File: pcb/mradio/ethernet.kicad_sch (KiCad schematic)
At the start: 28 parts, among them J1 JX0026D21BNL, U2 DP83825I, Y301 DSC1525JL2A-25M00000T

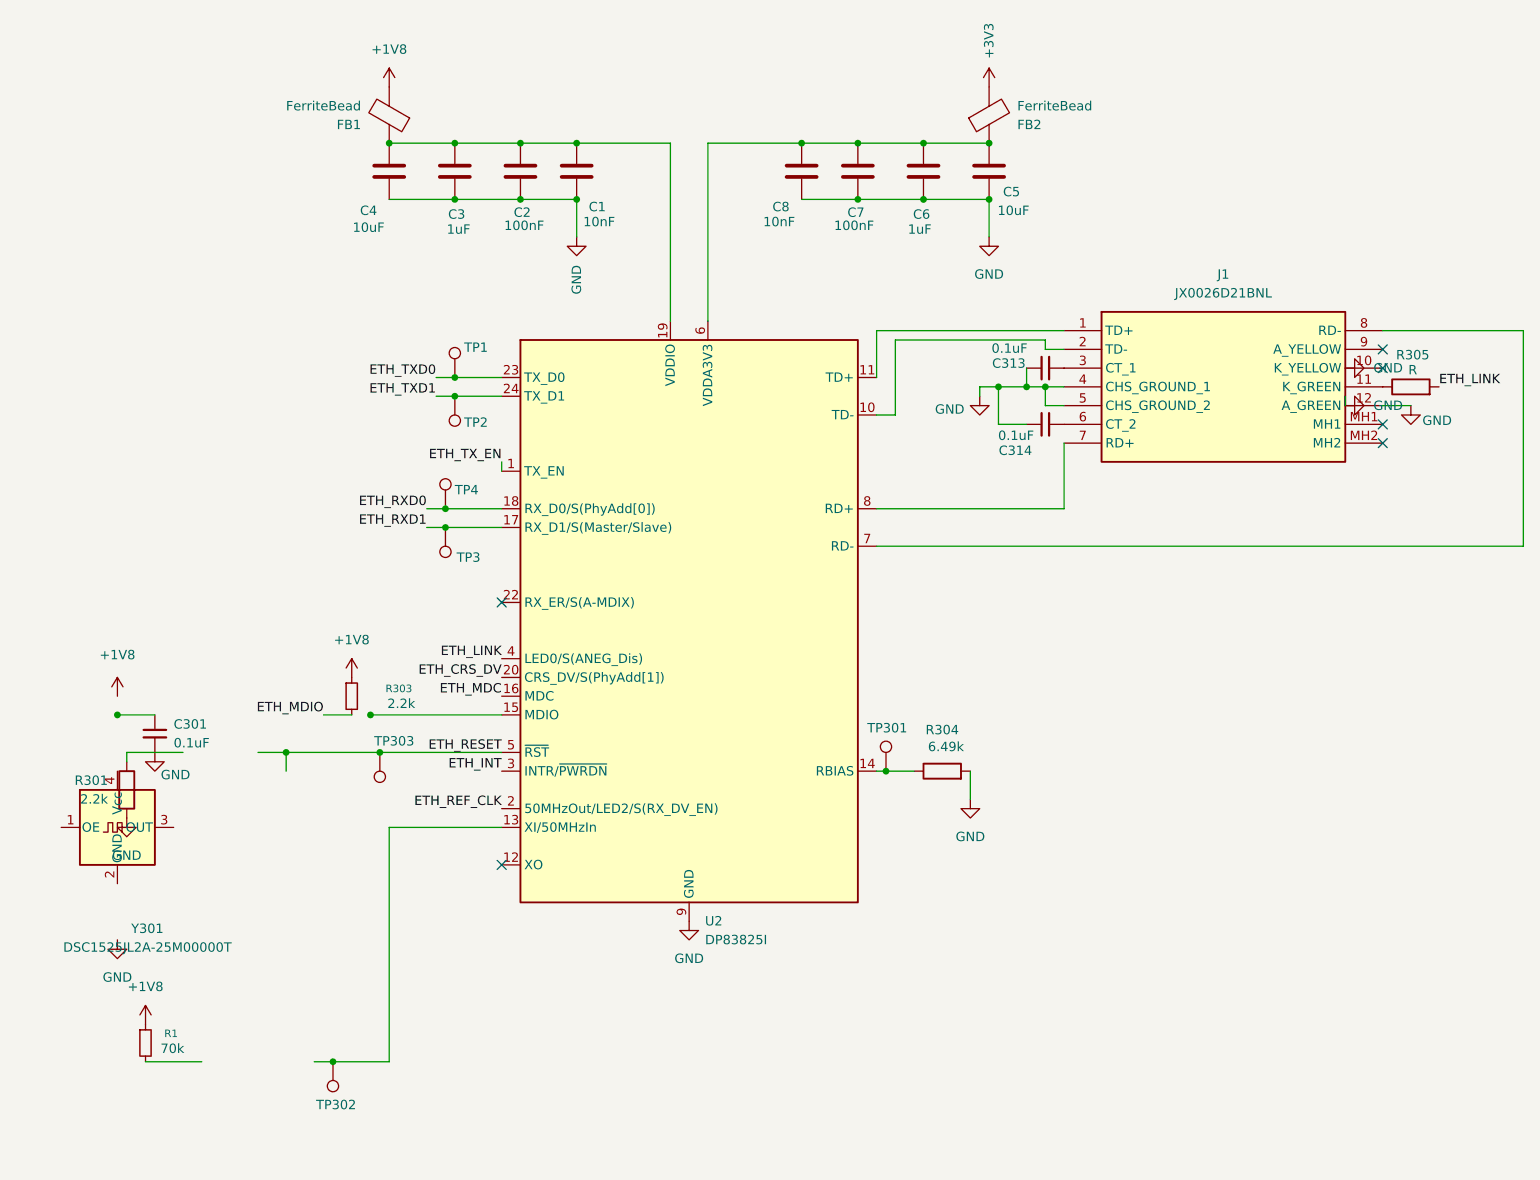
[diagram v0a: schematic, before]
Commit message: ethernet oscillator
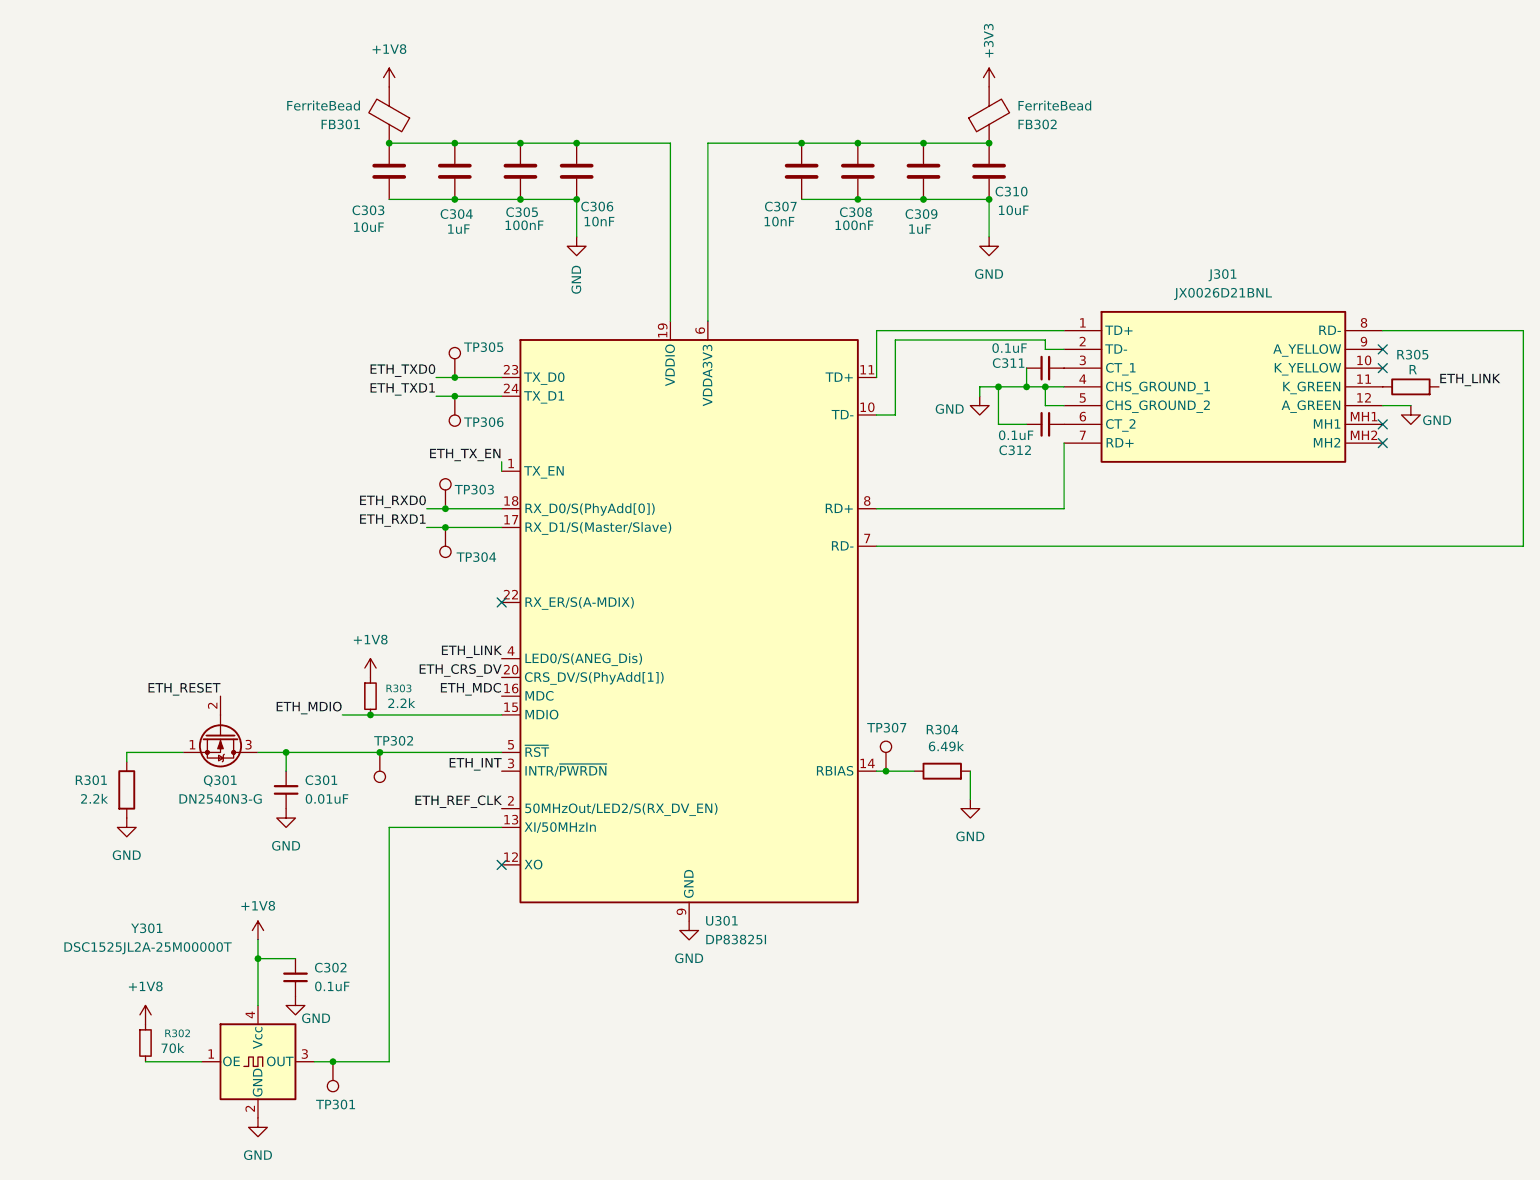
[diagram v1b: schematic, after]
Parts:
- added C301: 0.01uF, symbol Device:C_Small
- added Q301: DN2540N3-G, Package_TO_SOT_THT:TO-92_Inline, symbol Transistor_FET_Other:DN2540N3-G
- renumbered C301 to C302, C4 to C303, C3 to C304, C2 to C305, C1 to C306, C8 to C307, C7 to C308, C6 to C309, C5 to C310, C313 to C311, C314 to C312, FB1 to FB301, FB2 to FB302, J1 to J301, R1 to R302, TP302 to TP301, TP303 to TP302, TP4 to TP303, TP3 to TP304, TP1 to TP305, TP2 to TP306, TP301 to TP307, U2 to U301
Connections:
- net +1V8: now also C302.1, Y301.4 (Vcc)
- net ETH_MDIO: now also U301.15 (MDIO)
- net ETH_RESET: now also Q301.2 (G); no longer TP302.1, U301.5 (~{RST})
- net GND: now also Y301.2 (GND), C301.2
- net at R302.2: now also Y301.1 (OE)
- net at TP301.1, U301.13 (XI/50MHzIn): now also Y301.3 (OUT)
- net at R301.1: now also Q301.1 (S)
- new net: C301.1, Q301.3 (D), TP302.1, U301.5 (~{RST})
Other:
- moved on the sheet: C302, R303, Y301

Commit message: Fixed numbers
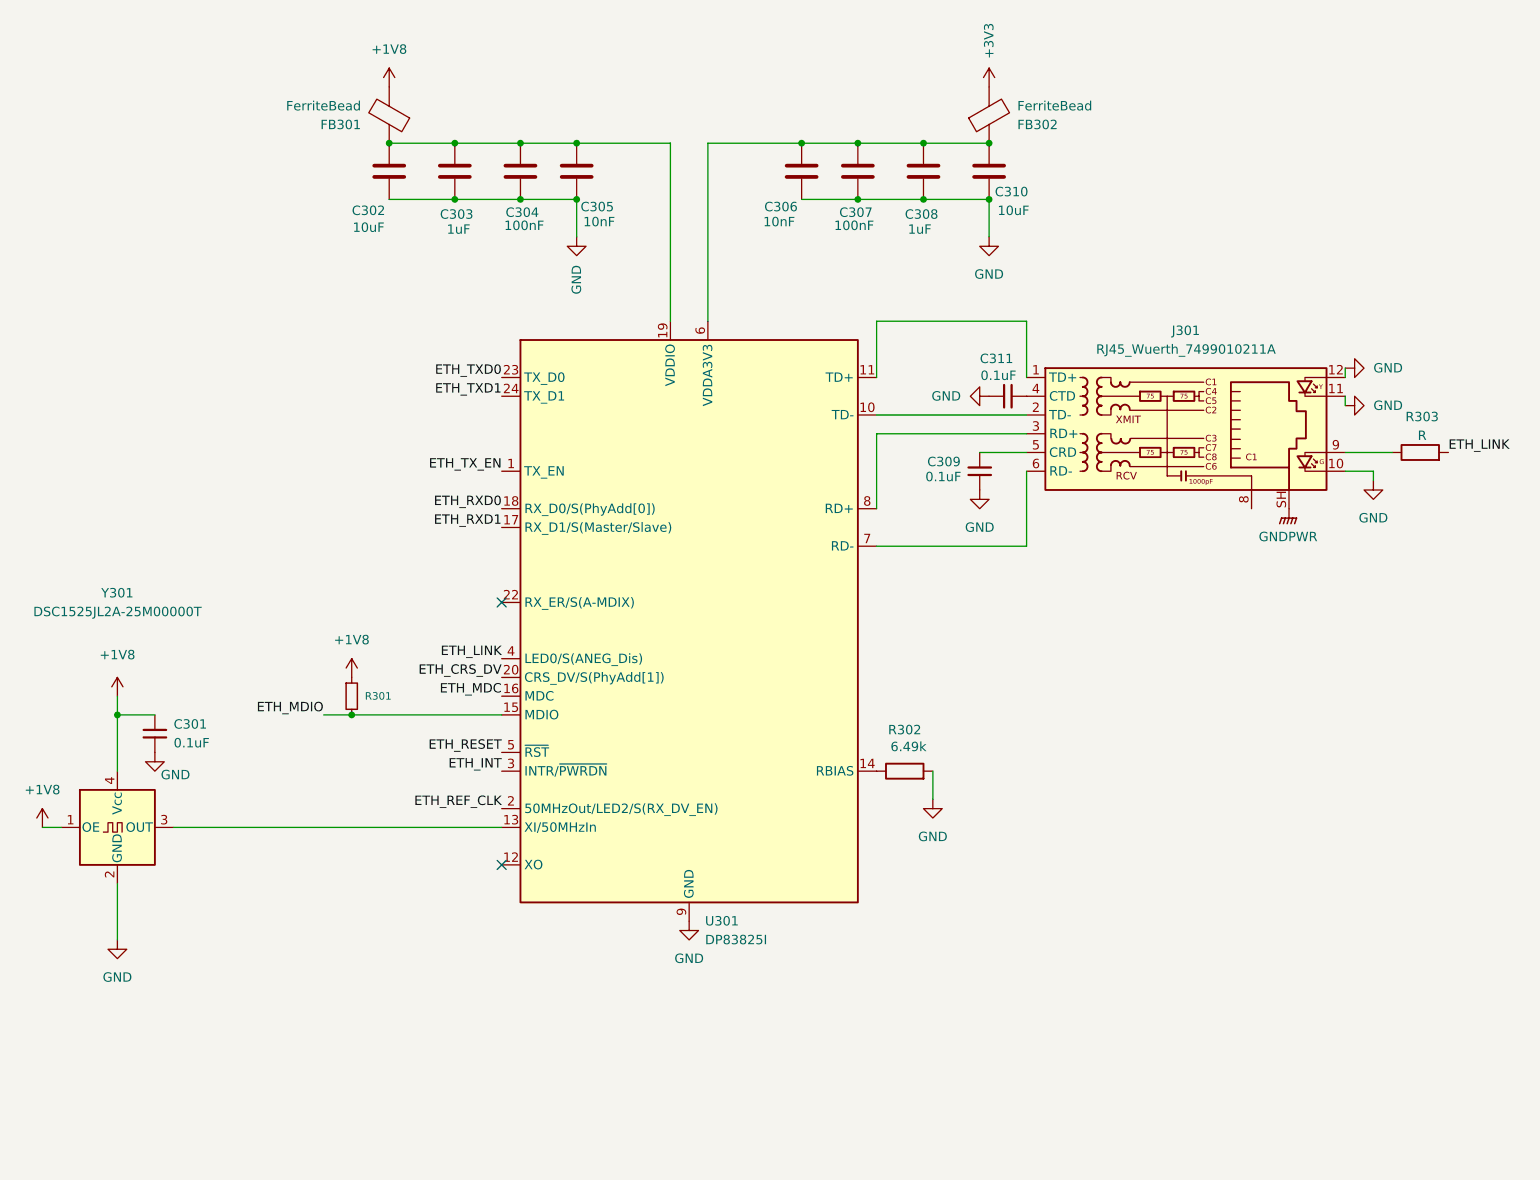
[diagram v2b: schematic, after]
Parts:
- removed C301: 0.01uF, symbol Device:C_Small
- removed C312: 0.1uF, symbol Device:C_Small
- removed J301: JX0026D21BNL, JX0026D21BNL:JX0026D21BNL, symbol symbols:JX0026D21BNL
- removed Q301: DN2540N3-G, Package_TO_SOT_THT:TO-92_Inline, symbol Transistor_FET_Other:DN2540N3-G
- removed R301: 2.2k, Package_TO_SOT_THT:TO-92_Inline, symbol Device:R
- removed R302: 70k, symbol Device:R_Small
- removed R305: R, symbol Device:R
- removed TP301, TP302, TP303, TP304, TP305, TP306, TP307: TestPoint, symbol Connector:TestPoint
- added C309: 0.1uF, symbol Device:C_Small
- added J301: RJ45_Wuerth_7499010211A, Connector_RJ:RJ45_Wuerth_7499010211A_Horizontal, symbol Connector:RJ45_Wuerth_7499010211A
- added R303: R, symbol Device:R
- R301: renamed from R303; value 2.2k -> (none)
- renumbered C302 to C301, C303 to C302, C304 to C303, C305 to C304, C306 to C305, C307 to C306, C308 to C307, C309 to C308, R304 to R302
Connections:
- net +1V8: now also Y301.1 (OE)
- net ETH_LINK: now also R303.2
- net ETH_RESET: now also U301.5 (~{RST})
- net GND: now also C309.2, J301.10, J301.11, J301.12
- net at U301.11 (TD+): now also J301.1 (TD+)
- net at U301.10 (TD-): now also J301.2 (TD-)
- net at C311.2: now also J301.4 (CTD)
- net at U301.8 (RD+): now also J301.3 (RD+)
- net at U301.7 (RD-): now also J301.6 (RD-)
- new net: C309.1, J301.5 (CRD)
- new net: J301.9, R303.1
- new net GNDPWR: J301.SH
- no-connect marks 6 -> 2
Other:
- moved on the sheet: C301, R301, R302, Y301

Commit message: undid overwrite
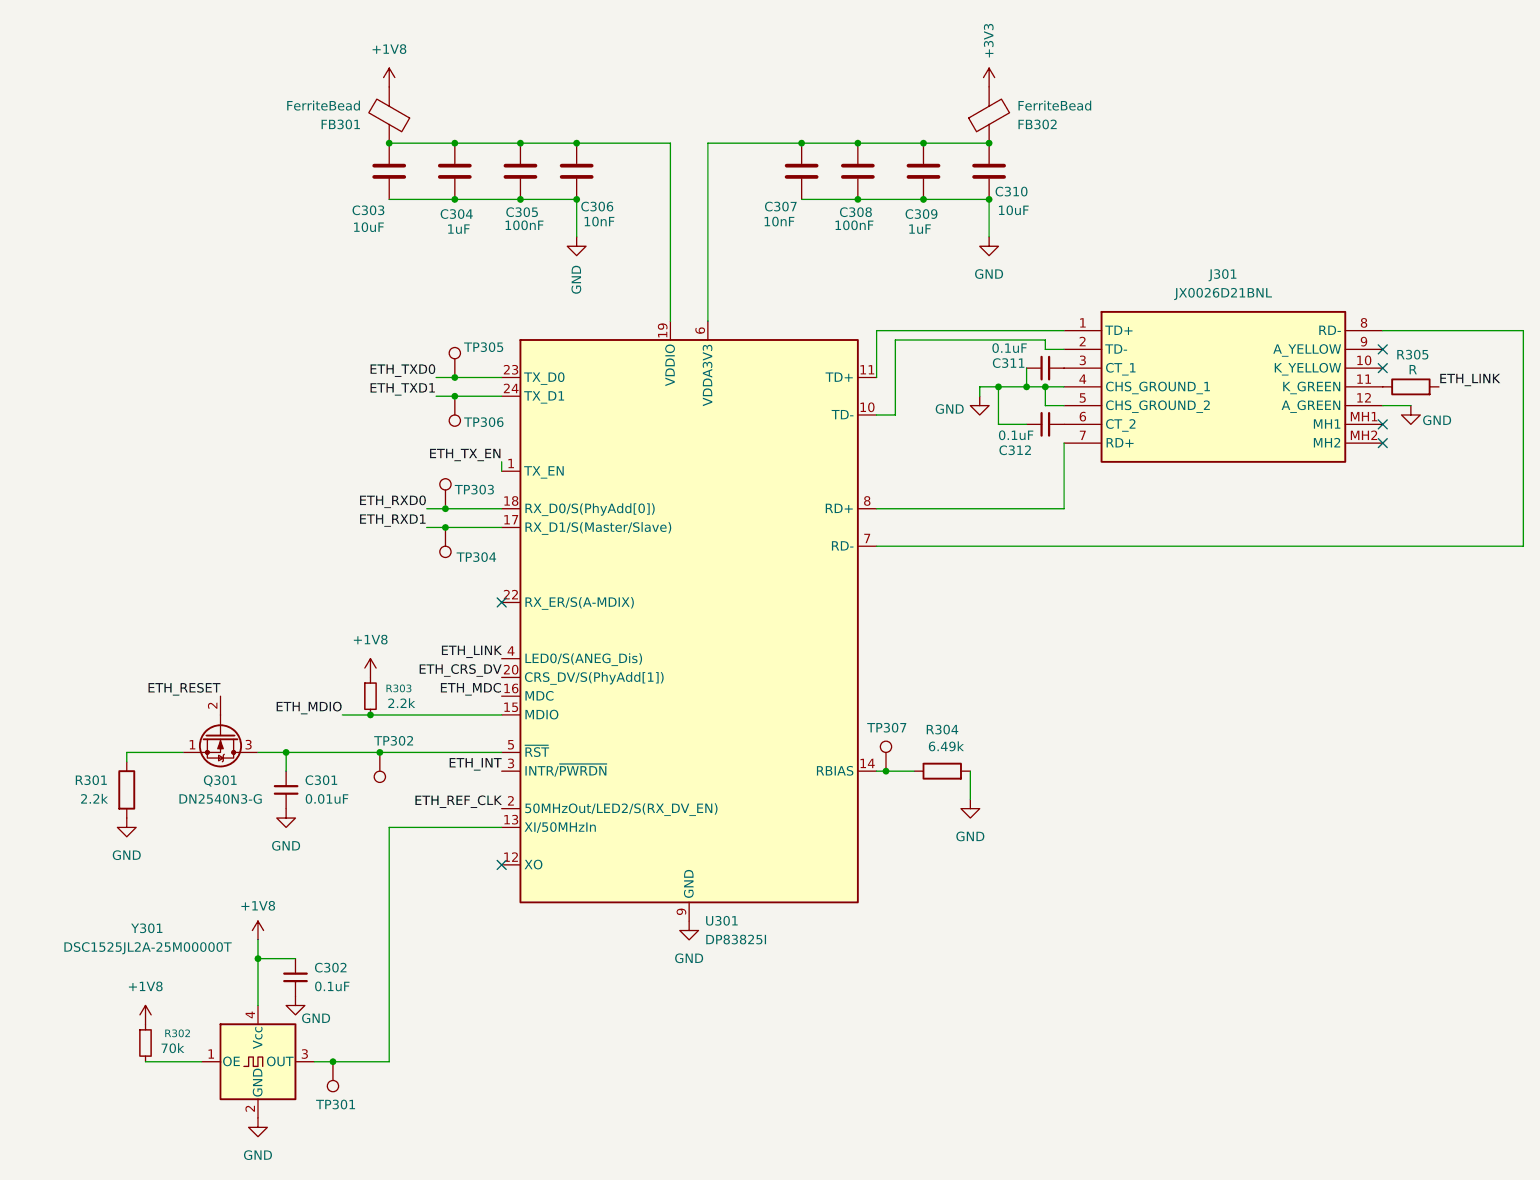
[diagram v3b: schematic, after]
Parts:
- removed C309: 0.1uF, symbol Device:C_Small
- removed J301: RJ45_Wuerth_7499010211A, Connector_RJ:RJ45_Wuerth_7499010211A_Horizontal, symbol Connector:RJ45_Wuerth_7499010211A
- removed R303: R, symbol Device:R
- added C301: 0.01uF, symbol Device:C_Small
- added C312: 0.1uF, symbol Device:C_Small
- added J301: JX0026D21BNL, JX0026D21BNL:JX0026D21BNL, symbol symbols:JX0026D21BNL
- added Q301: DN2540N3-G, Package_TO_SOT_THT:TO-92_Inline, symbol Transistor_FET_Other:DN2540N3-G
- added R301: 2.2k, Package_TO_SOT_THT:TO-92_Inline, symbol Device:R
- added R302: 70k, symbol Device:R_Small
- added R305: R, symbol Device:R
- added TP301, TP302, TP303, TP304, TP305, TP306, TP307: TestPoint, symbol Connector:TestPoint
- R303: renamed from R301; value (none) -> 2.2k
- renumbered C301 to C302, C302 to C303, C303 to C304, C304 to C305, C305 to C306, C306 to C307, C307 to C308, C308 to C309, R302 to R304
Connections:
- net +1V8: now also R302.1; no longer Y301.1 (OE)
- net ETH_LINK: now also R305.2
- net ETH_RESET: now also Q301.2 (G); no longer U301.5 (~{RST})
- net ETH_RXD0: now also TP303.1
- net ETH_RXD1: now also TP304.1
- net ETH_TXD0: now also TP305.1
- net ETH_TXD1: now also TP306.1
- net GND: now also C301.2, C312.1, J301.12 (A_GREEN), J301.4 (CHS_GROUND_1), J301.5 (CHS_GROUND_2), R301.2
- net at U301.11 (TD+): now also J301.1 (TD+)
- net at U301.10 (TD-): now also J301.2 (TD-)
- net at U301.8 (RD+): now also J301.7 (RD+)
- net at C311.2: now also J301.3 (CT_1)
- net at U301.7 (RD-): now also J301.8 (RD-)
- net at U301.13 (XI/50MHzIn), Y301.3 (OUT): now also TP301.1
- net at R304.1, U301.14 (RBIAS): now also TP307.1
- new net: Q301.1 (S), R301.1
- new net: C301.1, Q301.3 (D), TP302.1, U301.5 (~{RST})
- new net: R302.2, Y301.1 (OE)
- new net: J301.11 (K_GREEN), R305.1
- new net: C312.2, J301.6 (CT_2)
- no-connect marks 2 -> 6
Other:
- moved on the sheet: C302, R303, R304, Y301
